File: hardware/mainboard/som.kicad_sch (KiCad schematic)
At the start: 15 parts, among them SW1 SW_DIP_x04, U1 CP3225-100.000-3.3-25-X-T-TR, U2 AX3HAF1-135.0000T

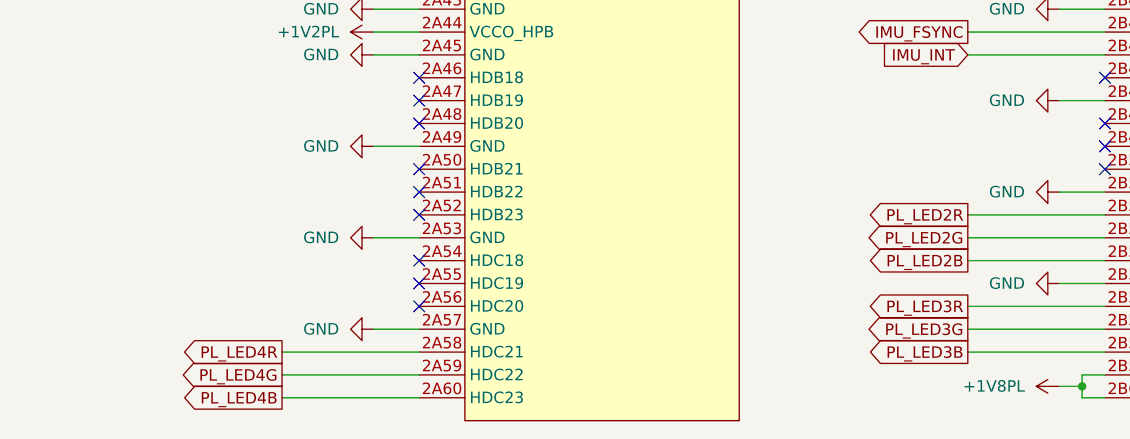
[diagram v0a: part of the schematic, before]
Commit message: Initial power routing
Signed-off-by: gatecat <gatecat@ds0.me>
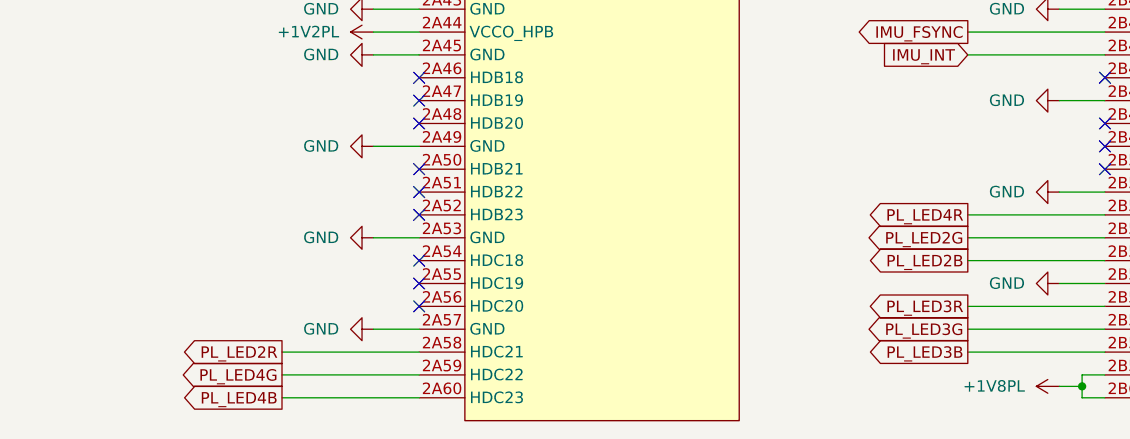
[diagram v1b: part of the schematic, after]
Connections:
- net PL_LED2R: now also SOM1.2A58 (HDC21); no longer SOM1.2B52 (HDC12)
- net PL_LED4R: now also SOM1.2B52 (HDC12); no longer SOM1.2A58 (HDC21)
